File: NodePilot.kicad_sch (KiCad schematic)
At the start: 38 parts, among them K1 SRD-05VDC-SL-C, Q1 2N3904, Q2 2N3904, Q4 2N3904, T1 1:1 600R, T2 1:1 600R, U1 PC817, U2 PC817, U3 B0505S-1WR2

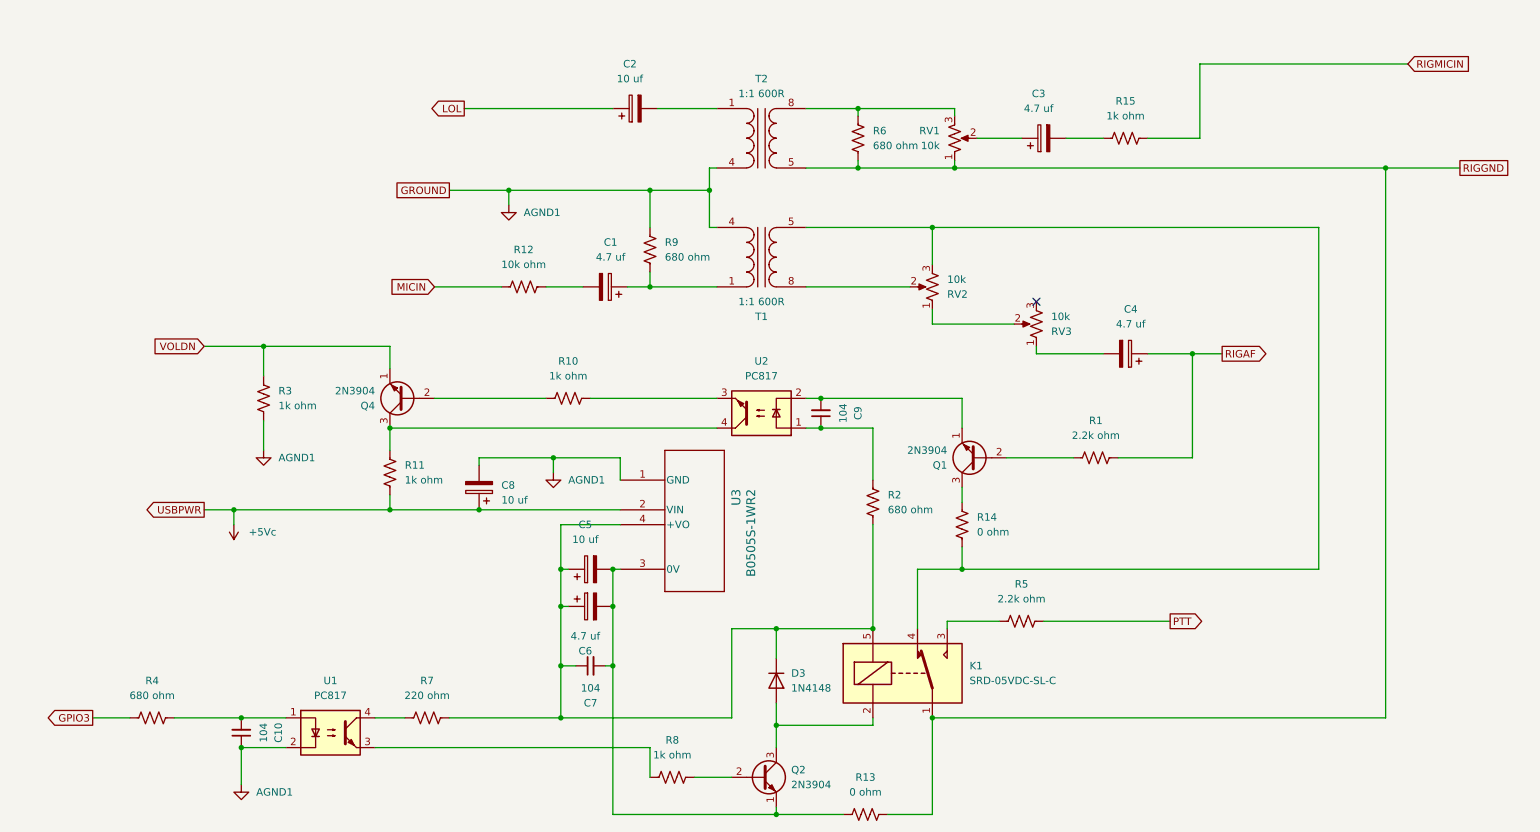
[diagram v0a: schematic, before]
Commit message: NodePilot Advanced
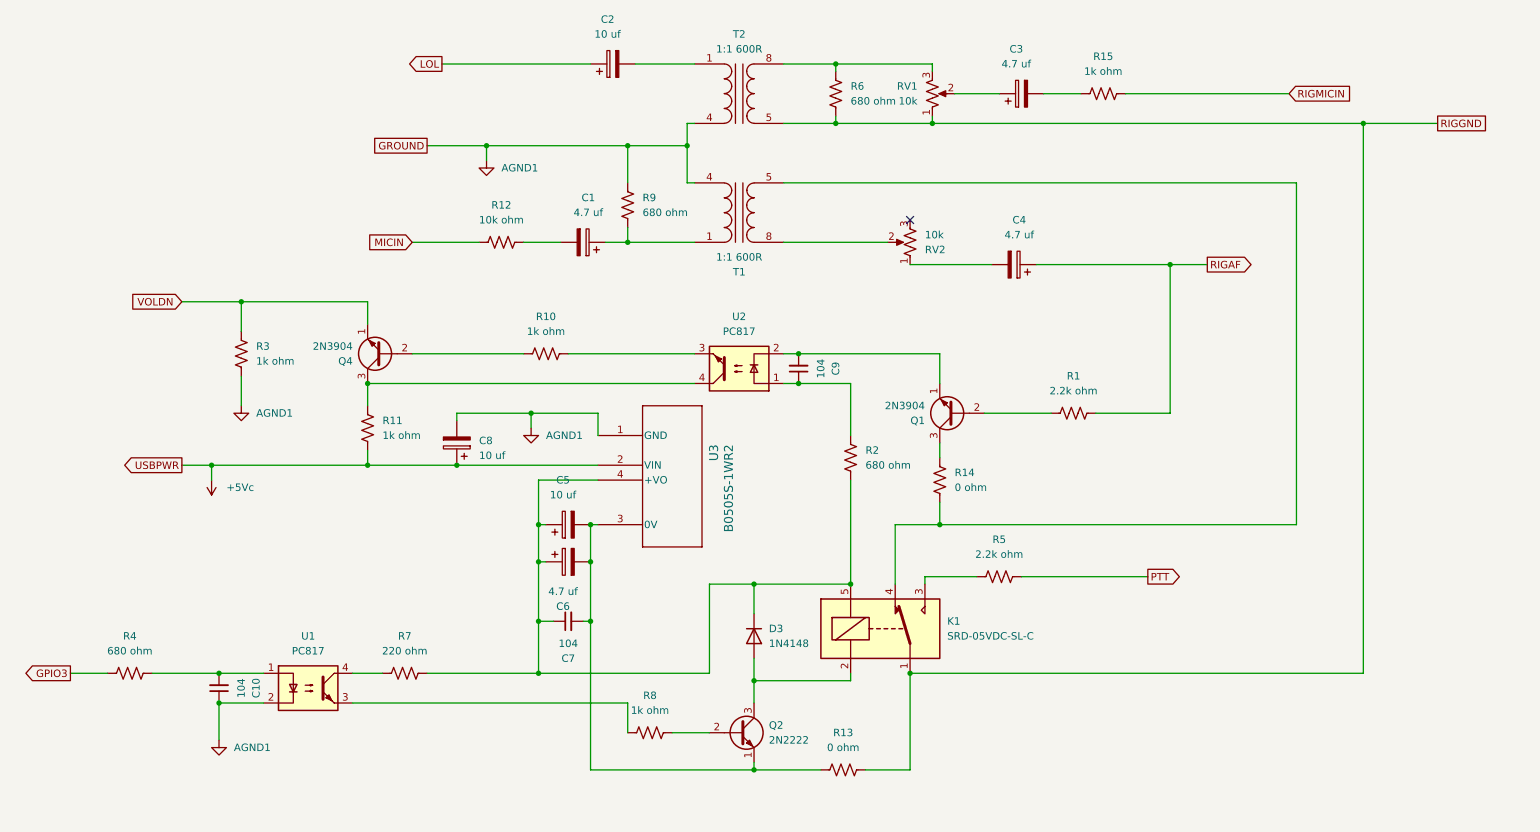
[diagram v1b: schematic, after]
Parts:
- removed RV3: 10k, symbol Device:R_Potentiometer_US
- Q2: value 2N3904 -> 2N2222
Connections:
- net at K1.4, R14.2, T1.5 (SA): no longer RV2.3
- net at RV2.1: now also C4.2
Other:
- title: NodePilot Remix By S21TIP -> NodePilot Advanced By S21TIP
- moved on the sheet: C1, C10, C2, C3, C4, C5, C6, C7, C8, C9, D3, K1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
